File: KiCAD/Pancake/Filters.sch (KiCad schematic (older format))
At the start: 19 parts, among them IC10 LF347N

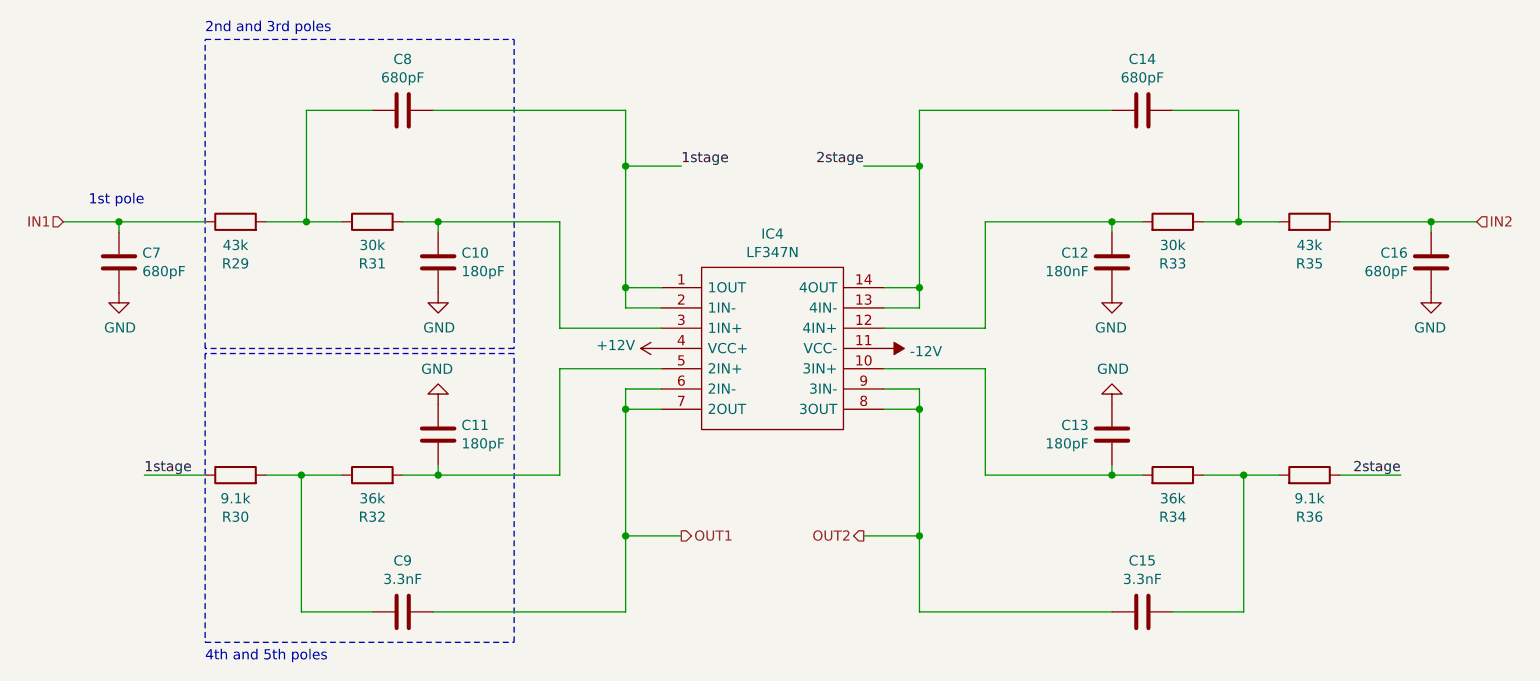
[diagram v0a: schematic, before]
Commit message: LED for connection of power. I was not able to find the footprint for the 1206 SMD LED that is in the Senior design lab, but I was able to find one for a similar model. With that being said, the model is the same but the specs are different. I believe this shouldn't be a problem as I just needed the Surface mount plates that could hold the LED from the Lab. Will add the Active low LED tomorrow , need to look at what pins I can use for LED and 5V.
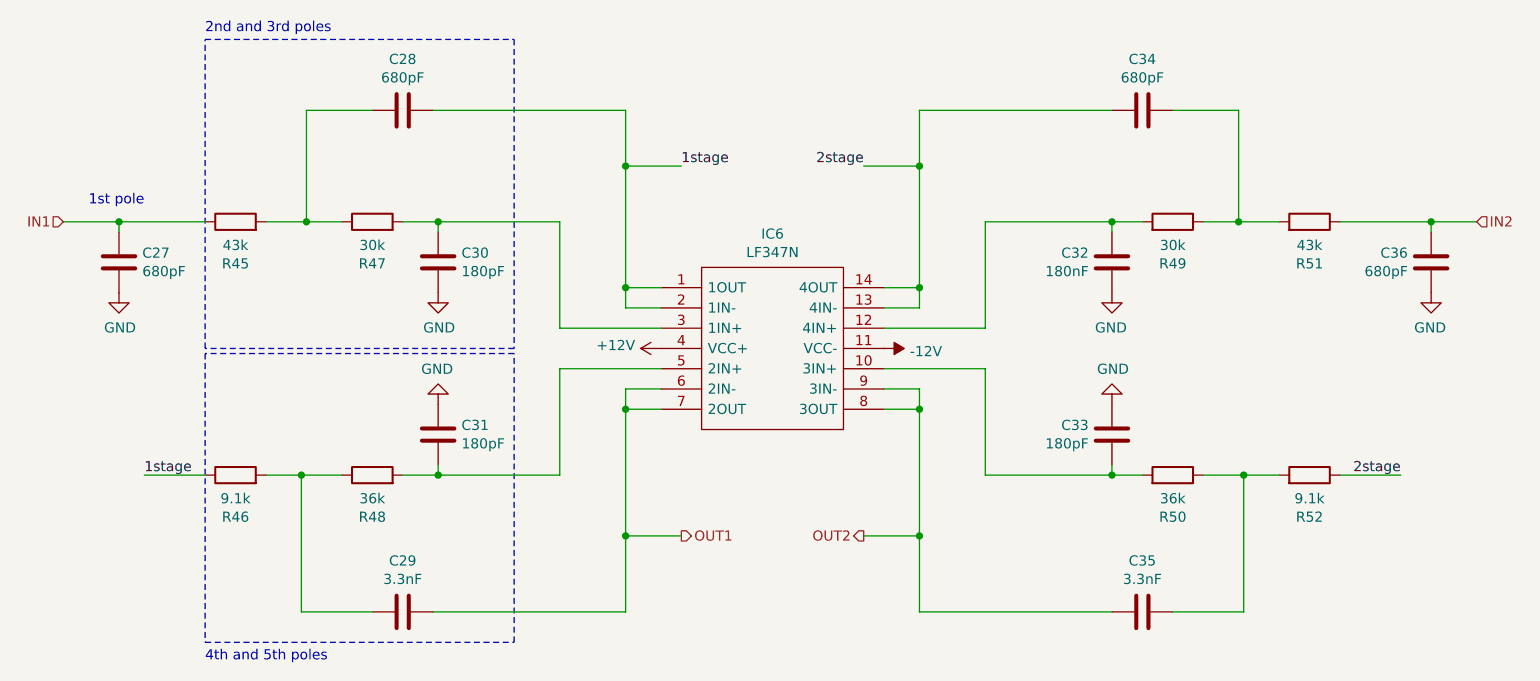
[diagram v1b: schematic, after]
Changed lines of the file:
@@
 AR Path="/61305DC1/610255EC" Ref="IC5"  Part="1"
 AR Path="/6133D86D/610255EC" Ref="IC4"  Part="1"
-F 0 "IC4" H 5875 3665 50  0000 C CNN
+F 0 "IC6" H 5875 3665 50  0000 C CNN
 F 1 "LF347N" H 5875 3574 50  0000 C CNN
 F 2 "SamacSys_Parts:DIP794W56P254L1905H533Q14N" H 6275 3500 50  0001 L CNN
@@
 AR Path="/61305DC1/6102CCC5" Ref="R37"  Part="1"
 AR Path="/6133D86D/6102CCC5" Ref="R29"  Part="1"
-F 0 "R29" V 3018 3075 50  0000 C CNN
+F 0 "R45" V 3018 3075 50  0000 C CNN
 F 1 "43k" V 3109 3075 50  0000 C CNN
 F 2 "Resistor_THT:R_Axial_DIN0207_L6.3mm_D2.5mm_P10.16mm_Horizontal" V 3155 3075 50  0001 C CNN
@@
 AR Path="/61305DC1/6102D406" Ref="R39"  Part="1"
 AR Path="/6133D86D/6102D406" Ref="R31"  Part="1"
-F 0 "R31" V 3693 3075 50  0000 C CNN
+F 0 "R47" V 3693 3075 50  0000 C CNN
 F 1 "30k" V 3784 3075 50  0000 C CNN
 F 2 "Resistor_THT:R_Axial_DIN0207_L6.3mm_D2.5mm_P10.16mm_Horizontal" V 3830 3075 50  0001 C CNN
@@
 AR Path="/61305DC1/6102D50F" Ref="C18"  Part="1"
 AR Path="/6133D86D/6102D50F" Ref="C8"  Part="1"
-F 0 "C8" V 3798 2525 50  0000 C CNN
+F 0 "C28" V 3798 2525 50  0000 C CNN
 F 1 "680pF" V 3889 2525 50  0000 C CNN
 F 2 "Capacitor_THT:C_Disc_D4.3mm_W1.9mm_P5.00mm" H 4088 2375 50  0001 C CNN
@@
 AR Path="/61305DC1/6102E9B3" Ref="C20"  Part="1"
 AR Path="/6133D86D/6102E9B3" Ref="C10"  Part="1"
-F 0 "C10" H 4110 3229 50  0000 R CNN
+F 0 "C30" H 4110 3229 50  0000 R CNN
 F 1 "180pF" H 4110 3320 50  0000 R CNN
 F 2 "Capacitor_THT:C_Disc_D4.3mm_W1.9mm_P5.00mm" H 4263 3125 50  0001 C CNN
@@
 AR Path="/61305DC1/6102F743" Ref="C17"  Part="1"
 AR Path="/6133D86D/6102F743" Ref="C7"  Part="1"
-F 0 "C7" H 2535 3229 50  0000 R CNN
+F 0 "C27" H 2535 3229 50  0000 R CNN
 F 1 "680pF" H 2535 3320 50  0000 R CNN
 F 2 "Capacitor_THT:C_Disc_D4.3mm_W1.9mm_P5.00mm" H 2688 3125 50  0001 C CNN
@@
 AR Path="/61305DC1/6103B127" Ref="R38"  Part="1"
 AR Path="/6133D86D/6103B127" Ref="R30"  Part="1"
-F 0 "R30" V 3018 4325 50  0000 C CNN
+F 0 "R46" V 3018 4325 50  0000 C CNN
 F 1 "9.1k" V 3109 4325 50  0000 C CNN
 F 2 "Resistor_THT:R_Axial_DIN0207_L6.3mm_D2.5mm_P10.16mm_Horizontal" V 3155 4325 50  0001 C CNN
@@
 AR Path="/61305DC1/6103B12D" Ref="R40"  Part="1"
 AR Path="/6133D86D/6103B12D" Ref="R32"  Part="1"
-F 0 "R32" V 3693 4325 50  0000 C CNN
+F 0 "R48" V 3693 4325 50  0000 C CNN
 F 1 "36k" V 3784 4325 50  0000 C CNN
 F 2 "Resistor_THT:R_Axial_DIN0207_L6.3mm_D2.5mm_P10.16mm_Horizontal" V 3830 4325 50  0001 C CNN
@@
 AR Path="/61305DC1/6103B133" Ref="C19"  Part="1"
 AR Path="/6133D86D/6103B133" Ref="C9"  Part="1"
-F 0 "C9" V 3798 5000 50  0000 C CNN
+F 0 "C29" V 3798 5000 50  0000 C CNN
 F 1 "3.3nF" V 3889 5000 50  0000 C CNN
 F 2 "Capacitor_THT:C_Disc_D4.3mm_W1.9mm_P5.00mm" H 4088 4850 50  0001 C CNN
@@
 AR Path="/61305DC1/6103B139" Ref="C21"  Part="1"
 AR Path="/6133D86D/6103B139" Ref="C11"  Part="1"
-F 0 "C11" H 4110 4079 50  0000 R CNN
+F 0 "C31" H 4110 4079 50  0000 R CNN
 F 1 "180pF" H 4110 4170 50  0000 R CNN
 F 2 "Capacitor_THT:C_Disc_D4.3mm_W1.9mm_P5.00mm" H 4263 3975 50  0001 C CNN
@@
 AR Path="/61305DC1/610910A4" Ref="R43"  Part="1"
 AR Path="/6133D86D/610910A4" Ref="R35"  Part="1"
-F 0 "R35" V 8318 3075 50  0000 C CNN
+F 0 "R51" V 8318 3075 50  0000 C CNN
 F 1 "43k" V 8409 3075 50  0000 C CNN
 F 2 "Resistor_THT:R_Axial_DIN0207_L6.3mm_D2.5mm_P10.16mm_Horizontal" V 8455 3075 50  0001 C CNN
@@
 AR Path="/61305DC1/610910AA" Ref="R41"  Part="1"
 AR Path="/6133D86D/610910AA" Ref="R33"  Part="1"
-F 0 "R33" V 7643 3075 50  0000 C CNN
+F 0 "R49" V 7643 3075 50  0000 C CNN
 F 1 "30k" V 7734 3075 50  0000 C CNN
 F 2 "Resistor_THT:R_Axial_DIN0207_L6.3mm_D2.5mm_P10.16mm_Horizontal" V 7780 3075 50  0001 C CNN
@@
 AR Path="/61305DC1/610910B0" Ref="C24"  Part="1"
 AR Path="/6133D86D/610910B0" Ref="C14"  Part="1"
-F 0 "C14" V 7448 2525 50  0000 C CNN
+F 0 "C34" V 7448 2525 50  0000 C CNN
 F 1 "680pF" V 7539 2525 50  0000 C CNN
 F 2 "Capacitor_THT:C_Disc_D4.3mm_W1.9mm_P5.00mm" H 7738 2375 50  0001 C CNN
@@
 AR Path="/61305DC1/610910BC" Ref="C26"  Part="1"
 AR Path="/6133D86D/610910BC" Ref="C16"  Part="1"
-F 0 "C16" H 9010 3229 50  0000 R CNN
+F 0 "C36" H 9010 3229 50  0000 R CNN
 F 1 "680pF" H 9010 3320 50  0000 R CNN
 F 2 "Capacitor_THT:C_Disc_D4.3mm_W1.9mm_P5.00mm" H 9163 3125 50  0001 C CNN
@@
 AR Path="/61305DC1/610910E5" Ref="R44"  Part="1"
 AR Path="/6133D86D/610910E5" Ref="R36"  Part="1"
-F 0 "R36" V 8318 4325 50  0000 C CNN
+F 0 "R52" V 8318 4325 50  0000 C CNN
 F 1 "9.1k" V 8409 4325 50  0000 C CNN
 F 2 "Resistor_THT:R_Axial_DIN0207_L6.3mm_D2.5mm_P10.16mm_Horizontal" V 8455 4325 50  0001 C CNN
@@
 AR Path="/61305DC1/610910EB" Ref="R42"  Part="1"
 AR Path="/6133D86D/610910EB" Ref="R34"  Part="1"
-F 0 "R34" V 7643 4325 50  0000 C CNN
+F 0 "R50" V 7643 4325 50  0000 C CNN
 F 1 "36k" V 7734 4325 50  0000 C CNN
 F 2 "Resistor_THT:R_Axial_DIN0207_L6.3mm_D2.5mm_P10.16mm_Horizontal" V 7780 4325 50  0001 C CNN
@@
 AR Path="/61305DC1/610910F1" Ref="C25"  Part="1"
 AR Path="/6133D86D/610910F1" Ref="C15"  Part="1"
-F 0 "C15" V 7448 5000 50  0000 C CNN
+F 0 "C35" V 7448 5000 50  0000 C CNN
 F 1 "3.3nF" V 7539 5000 50  0000 C CNN
 F 2 "Capacitor_THT:C_Disc_D4.3mm_W1.9mm_P5.00mm" H 7738 4850 50  0001 C CNN
@@
 AR Path="/61305DC1/610910F7" Ref="C23"  Part="1"
 AR Path="/6133D86D/610910F7" Ref="C13"  Part="1"
-F 0 "C13" H 7435 4079 50  0000 R CNN
+F 0 "C33" H 7435 4079 50  0000 R CNN
 F 1 "180pF" H 7435 4170 50  0000 R CNN
 F 2 "Capacitor_THT:C_Disc_D4.3mm_W1.9mm_P5.00mm" H 7588 3975 50  0001 C CNN
@@
 AR Path="/61305DC1/610910B6" Ref="C22"  Part="1"
 AR Path="/6133D86D/610910B6" Ref="C12"  Part="1"
-F 0 "C12" H 7435 3229 50  0000 R CNN
+F 0 "C32" H 7435 3229 50  0000 R CNN
 F 1 "180nF" H 7435 3320 50  0000 R CNN
 F 2 "Capacitor_THT:C_Disc_D4.3mm_W1.9mm_P5.00mm" H 7588 3125 50  0001 C CNN

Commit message: Will need to retrace in order to be built at SDSU.
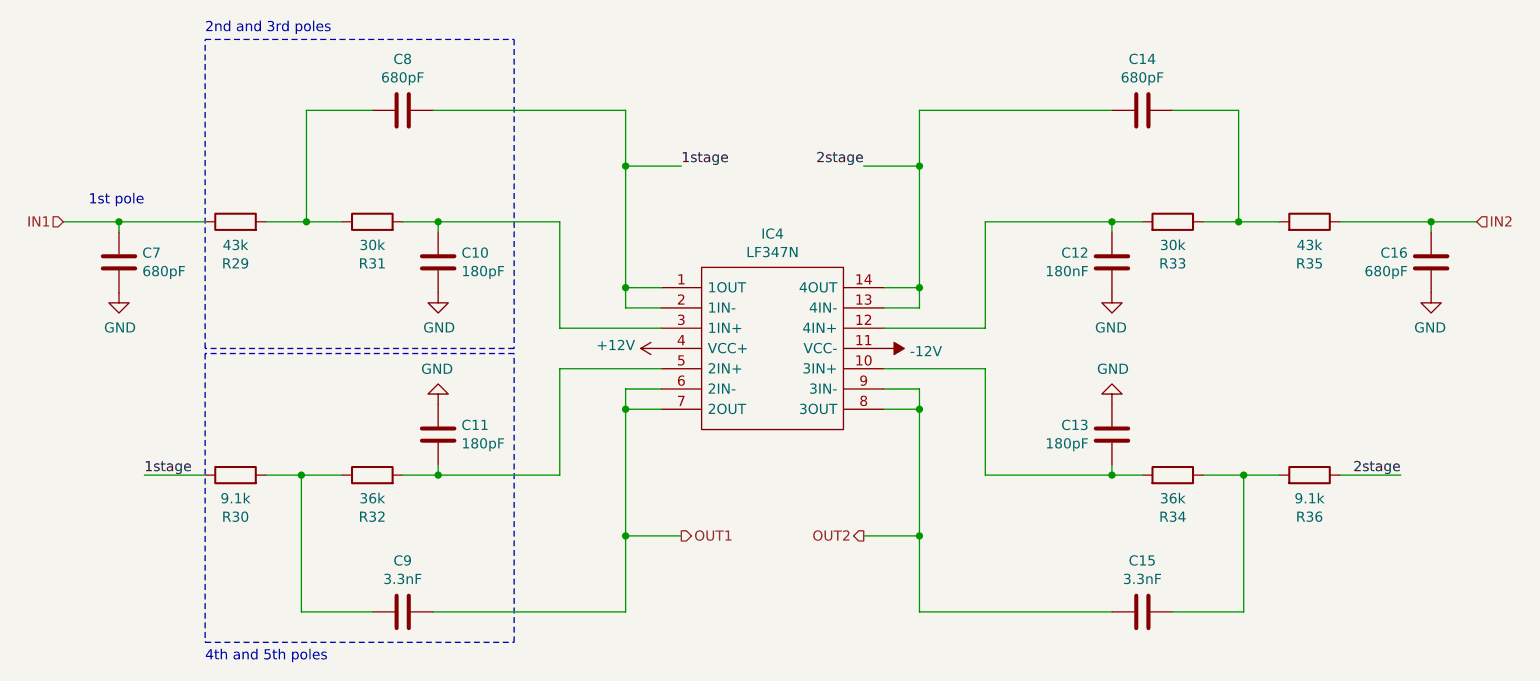
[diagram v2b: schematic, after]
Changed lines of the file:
@@
 AR Path="/61305DC1/610255EC" Ref="IC5"  Part="1"
 AR Path="/6133D86D/610255EC" Ref="IC4"  Part="1"
-F 0 "IC6" H 5875 3665 50  0000 C CNN
+F 0 "IC4" H 5875 3665 50  0000 C CNN
 F 1 "LF347N" H 5875 3574 50  0000 C CNN
 F 2 "SamacSys_Parts:DIP794W56P254L1905H533Q14N" H 6275 3500 50  0001 L CNN
@@
 AR Path="/61305DC1/6102CCC5" Ref="R37"  Part="1"
 AR Path="/6133D86D/6102CCC5" Ref="R29"  Part="1"
-F 0 "R45" V 3018 3075 50  0000 C CNN
+F 0 "R29" V 3018 3075 50  0000 C CNN
 F 1 "43k" V 3109 3075 50  0000 C CNN
 F 2 "Resistor_THT:R_Axial_DIN0207_L6.3mm_D2.5mm_P10.16mm_Horizontal" V 3155 3075 50  0001 C CNN
@@
 AR Path="/61305DC1/6102D406" Ref="R39"  Part="1"
 AR Path="/6133D86D/6102D406" Ref="R31"  Part="1"
-F 0 "R47" V 3693 3075 50  0000 C CNN
+F 0 "R31" V 3693 3075 50  0000 C CNN
 F 1 "30k" V 3784 3075 50  0000 C CNN
 F 2 "Resistor_THT:R_Axial_DIN0207_L6.3mm_D2.5mm_P10.16mm_Horizontal" V 3830 3075 50  0001 C CNN
@@
 AR Path="/61305DC1/6102D50F" Ref="C18"  Part="1"
 AR Path="/6133D86D/6102D50F" Ref="C8"  Part="1"
-F 0 "C28" V 3798 2525 50  0000 C CNN
+F 0 "C8" V 3798 2525 50  0000 C CNN
 F 1 "680pF" V 3889 2525 50  0000 C CNN
 F 2 "Capacitor_THT:C_Disc_D4.3mm_W1.9mm_P5.00mm" H 4088 2375 50  0001 C CNN
@@
 AR Path="/61305DC1/6102E9B3" Ref="C20"  Part="1"
 AR Path="/6133D86D/6102E9B3" Ref="C10"  Part="1"
-F 0 "C30" H 4110 3229 50  0000 R CNN
+F 0 "C10" H 4110 3229 50  0000 R CNN
 F 1 "180pF" H 4110 3320 50  0000 R CNN
 F 2 "Capacitor_THT:C_Disc_D4.3mm_W1.9mm_P5.00mm" H 4263 3125 50  0001 C CNN
@@
 AR Path="/61305DC1/6102F743" Ref="C17"  Part="1"
 AR Path="/6133D86D/6102F743" Ref="C7"  Part="1"
-F 0 "C27" H 2535 3229 50  0000 R CNN
+F 0 "C7" H 2535 3229 50  0000 R CNN
 F 1 "680pF" H 2535 3320 50  0000 R CNN
 F 2 "Capacitor_THT:C_Disc_D4.3mm_W1.9mm_P5.00mm" H 2688 3125 50  0001 C CNN
@@
 AR Path="/61305DC1/6103B127" Ref="R38"  Part="1"
 AR Path="/6133D86D/6103B127" Ref="R30"  Part="1"
-F 0 "R46" V 3018 4325 50  0000 C CNN
+F 0 "R30" V 3018 4325 50  0000 C CNN
 F 1 "9.1k" V 3109 4325 50  0000 C CNN
 F 2 "Resistor_THT:R_Axial_DIN0207_L6.3mm_D2.5mm_P10.16mm_Horizontal" V 3155 4325 50  0001 C CNN
@@
 AR Path="/61305DC1/6103B12D" Ref="R40"  Part="1"
 AR Path="/6133D86D/6103B12D" Ref="R32"  Part="1"
-F 0 "R48" V 3693 4325 50  0000 C CNN
+F 0 "R32" V 3693 4325 50  0000 C CNN
 F 1 "36k" V 3784 4325 50  0000 C CNN
 F 2 "Resistor_THT:R_Axial_DIN0207_L6.3mm_D2.5mm_P10.16mm_Horizontal" V 3830 4325 50  0001 C CNN
@@
 AR Path="/61305DC1/6103B133" Ref="C19"  Part="1"
 AR Path="/6133D86D/6103B133" Ref="C9"  Part="1"
-F 0 "C29" V 3798 5000 50  0000 C CNN
+F 0 "C9" V 3798 5000 50  0000 C CNN
 F 1 "3.3nF" V 3889 5000 50  0000 C CNN
 F 2 "Capacitor_THT:C_Disc_D4.3mm_W1.9mm_P5.00mm" H 4088 4850 50  0001 C CNN
@@
 AR Path="/61305DC1/6103B139" Ref="C21"  Part="1"
 AR Path="/6133D86D/6103B139" Ref="C11"  Part="1"
-F 0 "C31" H 4110 4079 50  0000 R CNN
+F 0 "C11" H 4110 4079 50  0000 R CNN
 F 1 "180pF" H 4110 4170 50  0000 R CNN
 F 2 "Capacitor_THT:C_Disc_D4.3mm_W1.9mm_P5.00mm" H 4263 3975 50  0001 C CNN
@@
 AR Path="/61305DC1/610910A4" Ref="R43"  Part="1"
 AR Path="/6133D86D/610910A4" Ref="R35"  Part="1"
-F 0 "R51" V 8318 3075 50  0000 C CNN
+F 0 "R35" V 8318 3075 50  0000 C CNN
 F 1 "43k" V 8409 3075 50  0000 C CNN
 F 2 "Resistor_THT:R_Axial_DIN0207_L6.3mm_D2.5mm_P10.16mm_Horizontal" V 8455 3075 50  0001 C CNN
@@
 AR Path="/61305DC1/610910AA" Ref="R41"  Part="1"
 AR Path="/6133D86D/610910AA" Ref="R33"  Part="1"
-F 0 "R49" V 7643 3075 50  0000 C CNN
+F 0 "R33" V 7643 3075 50  0000 C CNN
 F 1 "30k" V 7734 3075 50  0000 C CNN
 F 2 "Resistor_THT:R_Axial_DIN0207_L6.3mm_D2.5mm_P10.16mm_Horizontal" V 7780 3075 50  0001 C CNN
@@
 AR Path="/61305DC1/610910B0" Ref="C24"  Part="1"
 AR Path="/6133D86D/610910B0" Ref="C14"  Part="1"
-F 0 "C34" V 7448 2525 50  0000 C CNN
+F 0 "C14" V 7448 2525 50  0000 C CNN
 F 1 "680pF" V 7539 2525 50  0000 C CNN
 F 2 "Capacitor_THT:C_Disc_D4.3mm_W1.9mm_P5.00mm" H 7738 2375 50  0001 C CNN
@@
 AR Path="/61305DC1/610910BC" Ref="C26"  Part="1"
 AR Path="/6133D86D/610910BC" Ref="C16"  Part="1"
-F 0 "C36" H 9010 3229 50  0000 R CNN
+F 0 "C16" H 9010 3229 50  0000 R CNN
 F 1 "680pF" H 9010 3320 50  0000 R CNN
 F 2 "Capacitor_THT:C_Disc_D4.3mm_W1.9mm_P5.00mm" H 9163 3125 50  0001 C CNN
@@
 AR Path="/61305DC1/610910E5" Ref="R44"  Part="1"
 AR Path="/6133D86D/610910E5" Ref="R36"  Part="1"
-F 0 "R52" V 8318 4325 50  0000 C CNN
+F 0 "R36" V 8318 4325 50  0000 C CNN
 F 1 "9.1k" V 8409 4325 50  0000 C CNN
 F 2 "Resistor_THT:R_Axial_DIN0207_L6.3mm_D2.5mm_P10.16mm_Horizontal" V 8455 4325 50  0001 C CNN
@@
 AR Path="/61305DC1/610910EB" Ref="R42"  Part="1"
 AR Path="/6133D86D/610910EB" Ref="R34"  Part="1"
-F 0 "R50" V 7643 4325 50  0000 C CNN
+F 0 "R34" V 7643 4325 50  0000 C CNN
 F 1 "36k" V 7734 4325 50  0000 C CNN
 F 2 "Resistor_THT:R_Axial_DIN0207_L6.3mm_D2.5mm_P10.16mm_Horizontal" V 7780 4325 50  0001 C CNN
@@
 AR Path="/61305DC1/610910F1" Ref="C25"  Part="1"
 AR Path="/6133D86D/610910F1" Ref="C15"  Part="1"
-F 0 "C35" V 7448 5000 50  0000 C CNN
+F 0 "C15" V 7448 5000 50  0000 C CNN
 F 1 "3.3nF" V 7539 5000 50  0000 C CNN
 F 2 "Capacitor_THT:C_Disc_D4.3mm_W1.9mm_P5.00mm" H 7738 4850 50  0001 C CNN
@@
 AR Path="/61305DC1/610910F7" Ref="C23"  Part="1"
 AR Path="/6133D86D/610910F7" Ref="C13"  Part="1"
-F 0 "C33" H 7435 4079 50  0000 R CNN
+F 0 "C13" H 7435 4079 50  0000 R CNN
 F 1 "180pF" H 7435 4170 50  0000 R CNN
 F 2 "Capacitor_THT:C_Disc_D4.3mm_W1.9mm_P5.00mm" H 7588 3975 50  0001 C CNN
@@
 AR Path="/61305DC1/610910B6" Ref="C22"  Part="1"
 AR Path="/6133D86D/610910B6" Ref="C12"  Part="1"
-F 0 "C32" H 7435 3229 50  0000 R CNN
+F 0 "C12" H 7435 3229 50  0000 R CNN
 F 1 "180nF" H 7435 3320 50  0000 R CNN
 F 2 "Capacitor_THT:C_Disc_D4.3mm_W1.9mm_P5.00mm" H 7588 3125 50  0001 C CNN
